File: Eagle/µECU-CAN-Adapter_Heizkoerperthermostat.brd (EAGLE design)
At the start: 80 x 63.8 mm, 21 parts, among them IC1 MCP2515, IC2 PCA82C251, Q1 16MHz

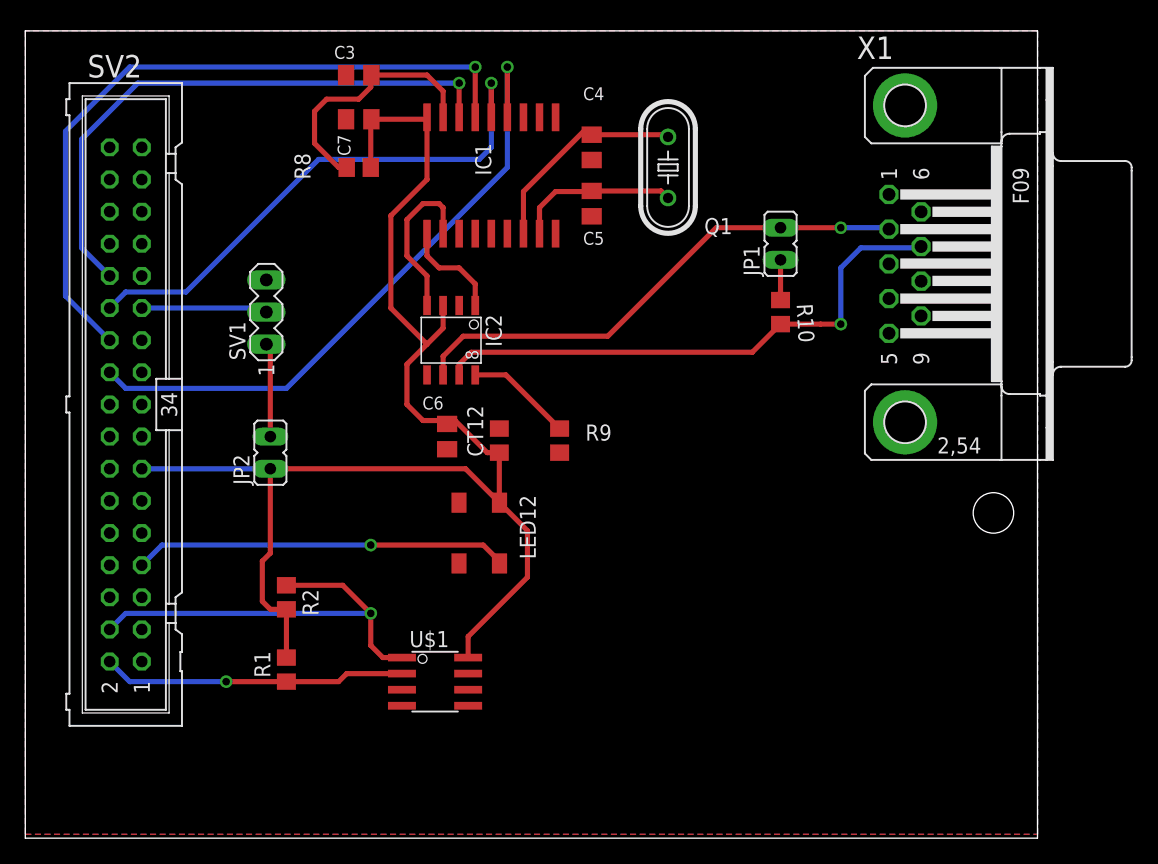
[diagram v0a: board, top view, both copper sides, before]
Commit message: rework board
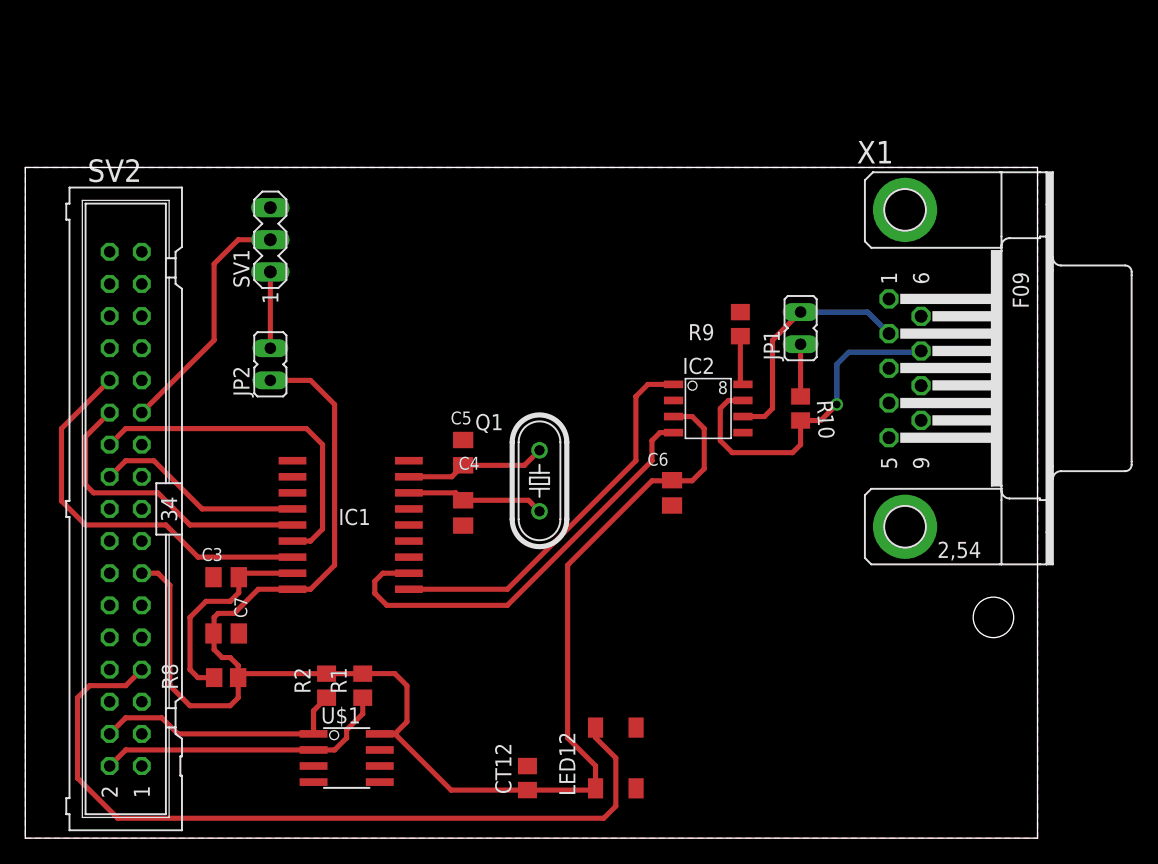
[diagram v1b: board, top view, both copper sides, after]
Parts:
- moved C7 42.0 mm to (15.9, 16.2), turned to 0 degrees
- moved R8 41.7 mm to (15.9, 12.7)
- moved C3 41.0 mm to (15.9, 20.6)
- moved C4 30.6 mm to (34.6, 25.7)
- moved IC1 29.8 mm to (25.7, 24.8), turned to 90 degrees
- moved Q1 26.8 mm to (40.6, 28.3), turned to 90 degrees
- moved CT12 26.8 mm to (39.7, 4.76)
- moved C5 22.2 mm to (34.6, 30.5), turned to 90 degrees
- moved LED12 20.8 mm to (46.7, 6.35), turned to 90 degrees
- moved IC2 20.3 mm to (54.0, 34.6), turned to 270 degrees
- moved C6 18.3 mm to (51.1, 27.3)
- moved R9 17.0 mm to (56.5, 40.6), turned to 270 degrees
- moved U$1 9.23 mm to (25.4, 6.35)
- moved X1 8.26 mm to (69.5, 37.1)
- moved SV2 8.25 mm to (7.94, 26.0)
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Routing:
- net PB5: track 51.1 -> 16.6 mm, vias 1 -> 0
- net PD2: track 29.6 -> 63.5 mm, vias 1 -> 0
- net PB4: track 56.4 -> 27.3 mm, vias 1 -> 0
- net N$10: track 41.3 -> 18.8 mm, vias 1 -> 0
- net N$7: track 8.18 -> 30.6 mm
- net N$6: track 13.0 -> 34.5 mm
- net PB3: track 43.2 -> 24.2 mm, vias 1 -> 0
- net +5V: track 111.9 -> 129.8 mm
- net N$8: track 43.8 -> 27.2 mm
- net PB2: track 46.1 -> 31.2 mm, vias 1 -> 0
- net PC4: track 34.2 -> 20.5 mm, vias 1 -> 0
- net PD6: track 9.97 -> 19.3 mm
- net N$3: track 16.9 -> 10.9 mm
- net N$5: track 8.43 -> 3.90 mm
- net N$4: track 20.3 -> 16.7 mm
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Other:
- board size 80 x 63.8 mm -> 80 x 53 mm
